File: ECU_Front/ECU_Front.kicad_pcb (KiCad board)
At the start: 2 copper layers, 100.5 x 54.9 mm, 19 parts, among them J1 Conn_01x04_Pin, J2 Conn_01x04_Pin, J3 Conn_01x02_Pin, U2 YAAJ_DCDC_StepDown_LM2596, U3 ESP32-DevKitC

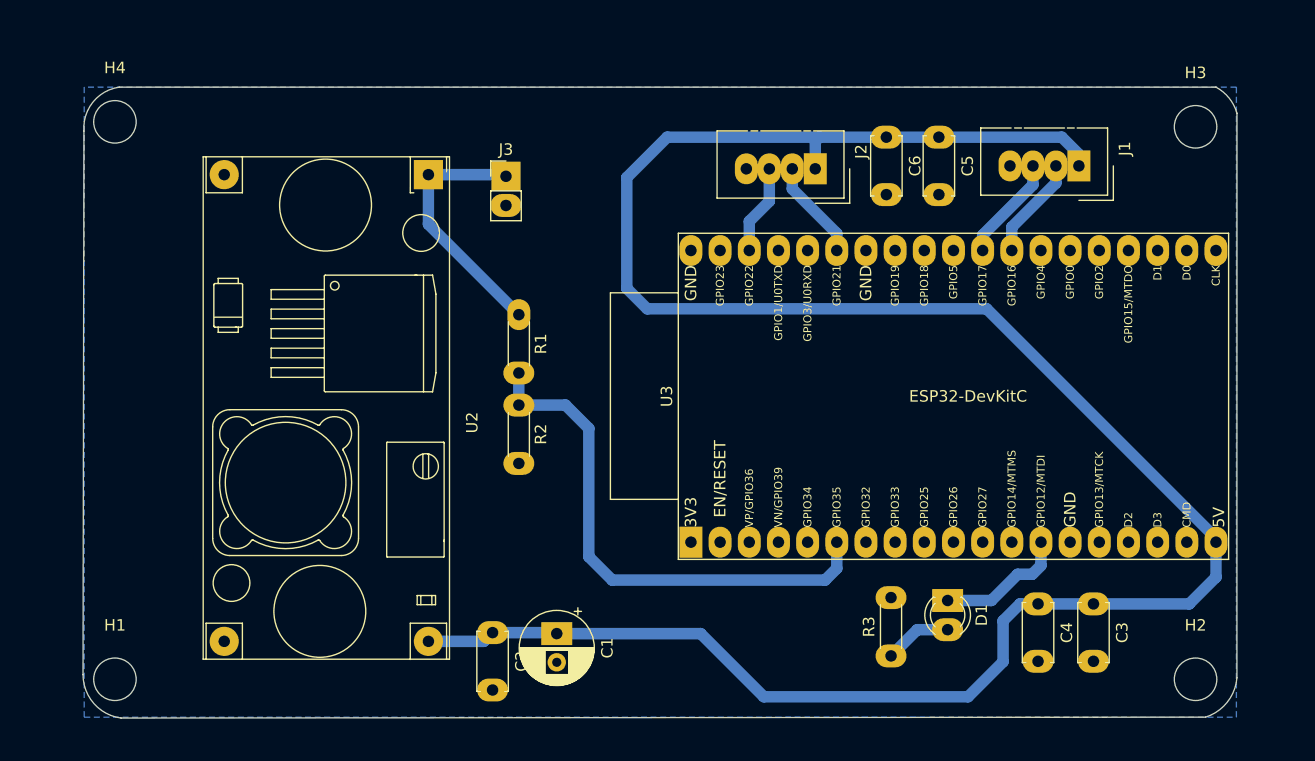
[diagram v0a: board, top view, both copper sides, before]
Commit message: final fix ECU Front
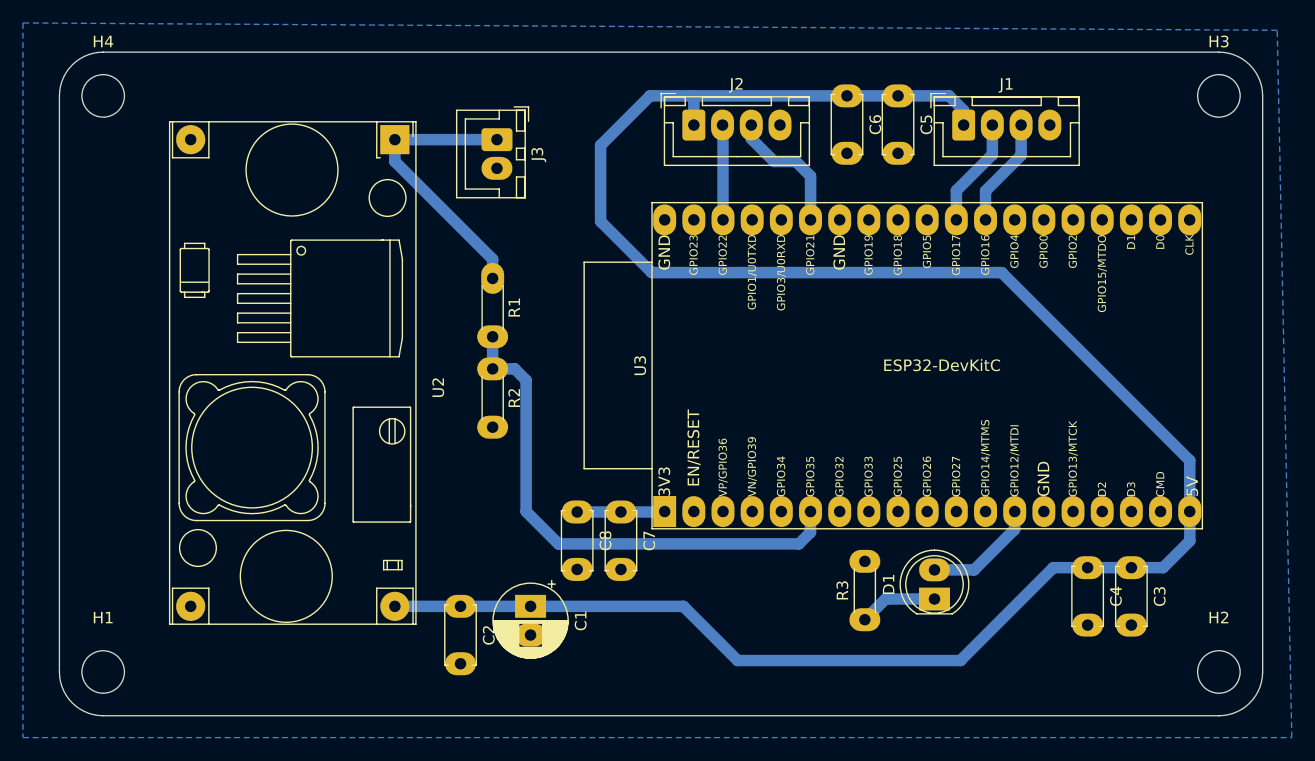
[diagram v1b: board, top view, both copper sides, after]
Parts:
- added C7: 10uF, Capacitor_THT:C_Disc_D5.0mm_W2.5mm_P5.00mm, F.Cu at (156.2, 122.6)
- added C8: 100nF, Capacitor_THT:C_Disc_D5.0mm_W2.5mm_P5.00mm, F.Cu at (152.4, 122.6)
- added G***: LOGO, LOGO, B.Cu at (126.4, 112.4)
- D1: footprint LED_THT:LED_D3.0mm_FlatTop -> LED_THT:LED_D5.0mm
- J1: value Conn_01x04_Pin -> Conn_display; footprint Connector:NS-Tech_Grove_1x04_P2mm_Vertical -> Connector_JST:JST_XH_B4B-XH-A_1x04_P2.50mm_Vertical
- J2: value Conn_01x04_Pin -> Conn_acc; footprint Connector:NS-Tech_Grove_1x04_P2mm_Vertical -> Connector_JST:JST_XH_B4B-XH-A_1x04_P2.50mm_Vertical
- J3: value Conn_01x02_Pin -> Conn_pwr; footprint Connector_PinHeader_2.54mm:PinHeader_1x02_P2.54mm_Vertical -> Connector_JST:JST_XH_B2B-XH-A_1x02_P2.50mm_Vertical
- U2: value YAAJ_DCDC_StepDown_LM2596 -> LM2596_buck
- moved J2 11.2 mm to (162.6, 88.9), turned to 0 degrees
- moved J1 10.6 mm to (186.1, 88.9), turned to 0 degrees
- moved C4 5.35 mm to (196.8, 127.4)
- moved C5 5.06 mm to (180.3, 86.4)
- moved C6 4.97 mm to (175.9, 86.4)
- moved C3 4.57 mm to (200.7, 127.4)
- moved U2 4.22 mm to (136.5, 90.2)
- moved R2 3.89 mm to (145.0, 110.1)
- moved R1 3.89 mm to (145.0, 102.3)
- moved R3 3.89 mm to (177.5, 132.0)
- moved C2 3.61 mm to (142.2, 130.8)
- moved U3 3.51 mm to (160.0, 122.6)
- moved H3 3.37 mm to (208.3, 86.4)
- moved C1 3.29 mm to (148.3, 130.8)
- moved J3 3.29 mm to (145.4, 90.2), turned to -90 degrees
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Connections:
- D1 pad 1: LED_ALIVE -> Net-(D1-K)
- D1 pad 2: Net-(D1-A) -> LED_ALIVE
- J1 pad 2: RXD2 -> TXD2
- J1 pad 3: TXD2 -> RXD2
- J2 pad 2: SDA -> SCL
- J2 pad 3: SCL -> SDA
- R3 pad 1: Net-(D1-A) -> Net-(D1-K)
- U3 pad 1: unconnected-(U3-3V3-Pad1) -> +3V3
- U3 pad 14: unconnected-(U3-GND-Pad14) -> GND
- U3 pad 38: unconnected-(U3-GND-Pad38) -> GND
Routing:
- net +5V: track 196.3 -> 186.8 mm
- net +3V3: track 0.00 -> 7.64 mm
- net Net-(D1-K): track 0.00 -> 6.81 mm
- net Net-(D1-A): track 5.87 -> 0.00 mm
- net SDA: track 8.72 -> 11.5 mm
- net +12V: track 22.3 -> 24.5 mm
- net LED_ALIVE: track 11.4 -> 10.00 mm
- net RXD2: track 8.96 -> 9.54 mm
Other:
- board size 100.5 x 54.9 mm -> 104.8 x 57.8 mm
